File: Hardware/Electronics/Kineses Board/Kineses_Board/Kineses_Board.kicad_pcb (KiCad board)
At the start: 2 copper layers, 26 x 65.6 mm, 19 parts, among them J1 Barrel_Jack, J2 Thumb, J3 Index, J4 Middle, J5 Ring, J6 Pinky, J7 Wrist, J8 HC-05

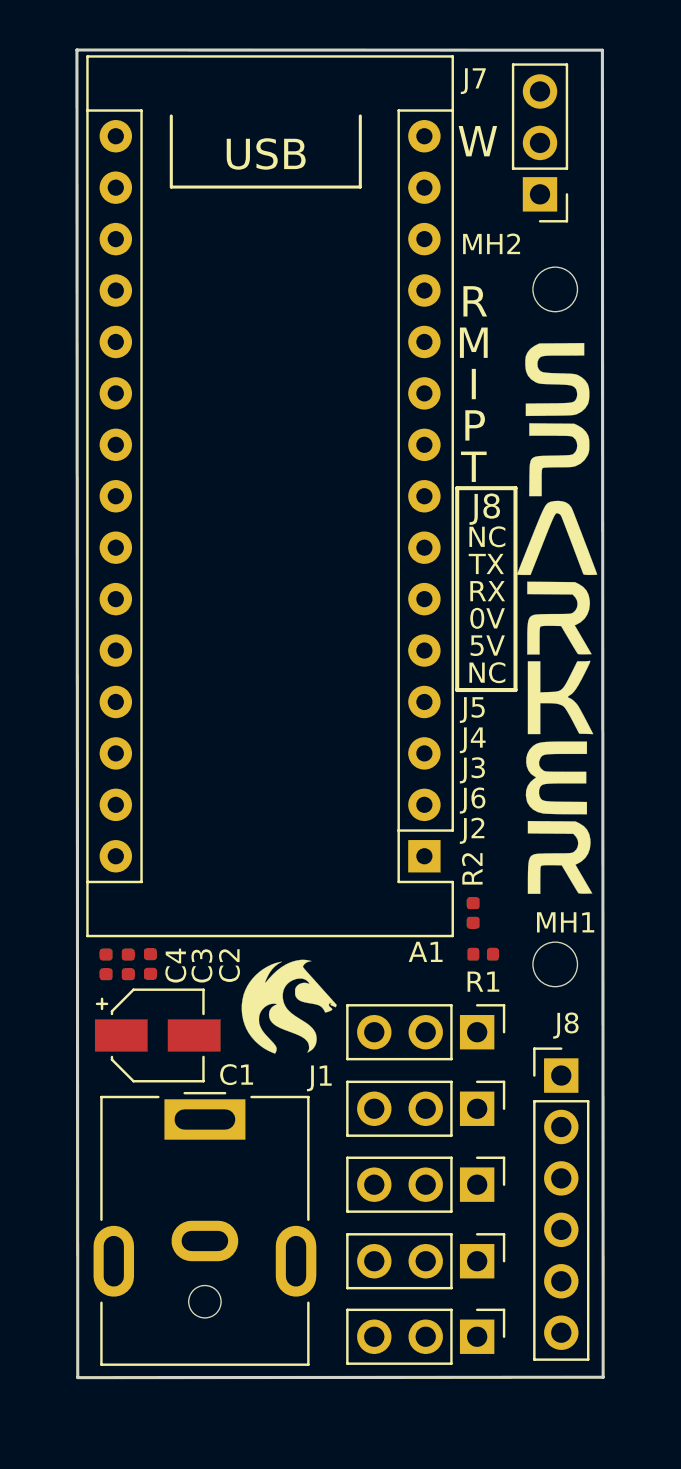
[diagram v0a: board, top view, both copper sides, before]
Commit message: Finished routing
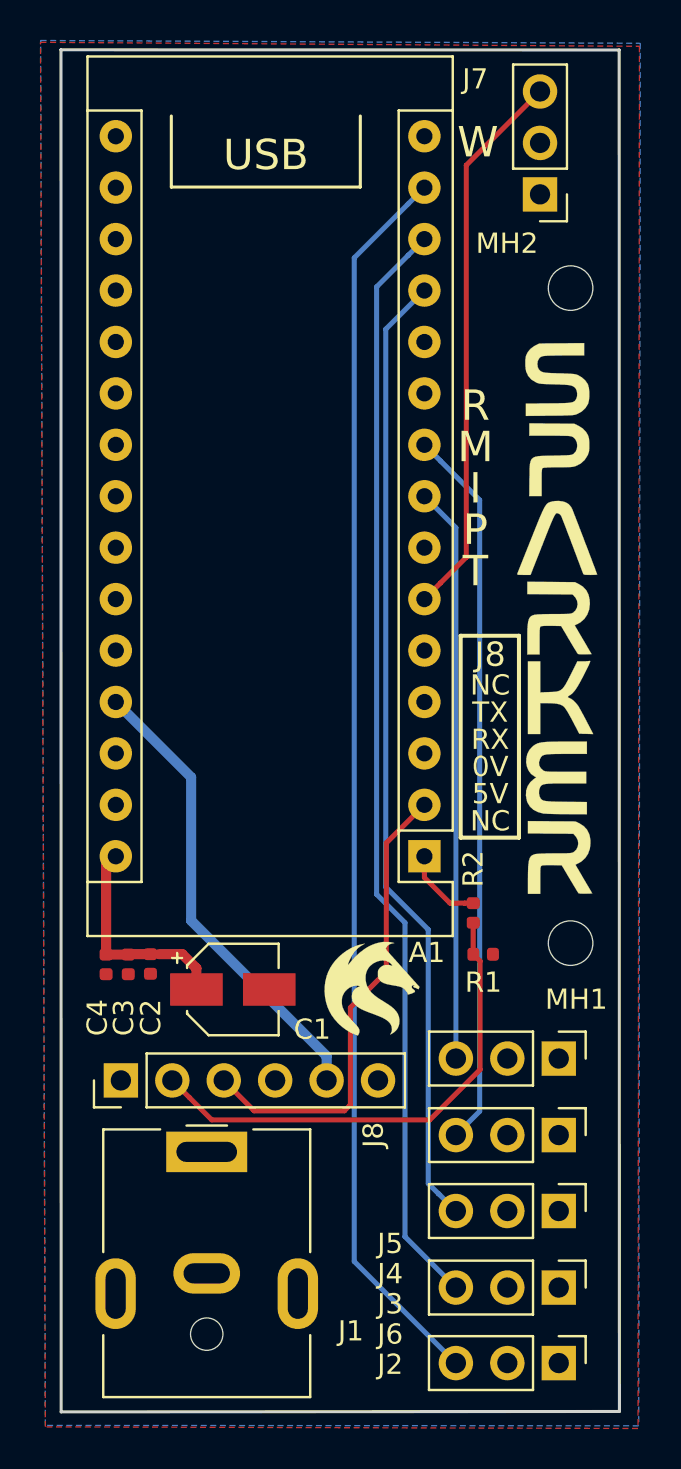
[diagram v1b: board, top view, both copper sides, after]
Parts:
- moved J8 21.8 mm to (137.0, 102.7), turned to 90 degrees
- moved C1 4.35 mm to (142.6, 98.2)
- moved J3 4.23 mm to (158.6, 109.1)
- moved J4 4.23 mm to (158.6, 105.4)
- moved J6 4.23 mm to (158.6, 112.9)
- moved J2 4.23 mm to (158.6, 116.6)
- moved J5 4.23 mm to (158.6, 101.6)
- moved LOGO2 4.19 mm to (149.4, 98.2)
- moved J1 1.60 mm to (141.3, 106.2)
- moved MH1 1.30 mm to (159.2, 95.9)
- moved MH2 0.76 mm to (159.2, 63.5)
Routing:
- net /Thumb: track 0.00 -> 61.6 mm
- net /Pinky: track 0.00 -> 54.4 mm
- net /Index: track 0.00 -> 47.7 mm
- net /Middle: track 0.00 -> 35.7 mm
- net /Ring: track 0.00 -> 28.4 mm
- net /Wrist: track 0.00 -> 27.4 mm
- net /TX: track 0.00 -> 24.4 mm
- net /RX: track 0.00 -> 23.3 mm
- net /+5V: track 0.00 -> 23.0 mm
- net /VIN: track 0.00 -> 10.9 mm
- net Net-(A1-Pad1): track 0.00 -> 3.98 mm
- added copper zone on F.Cu, net /GND
- added copper zone on B.Cu, net /VIN
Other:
- board size 26 x 65.6 mm -> 27.6 x 67.3 mm
